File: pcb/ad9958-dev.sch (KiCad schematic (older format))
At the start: 88 parts, among them J2 5V, J3 OUT0, J4 OUT1, J5 HEAD-M10X2, U1 LM1117-1v8-SOT223, U2 LMH6714, U3 AD9958, U4 LMH6714, X1 25 MHz

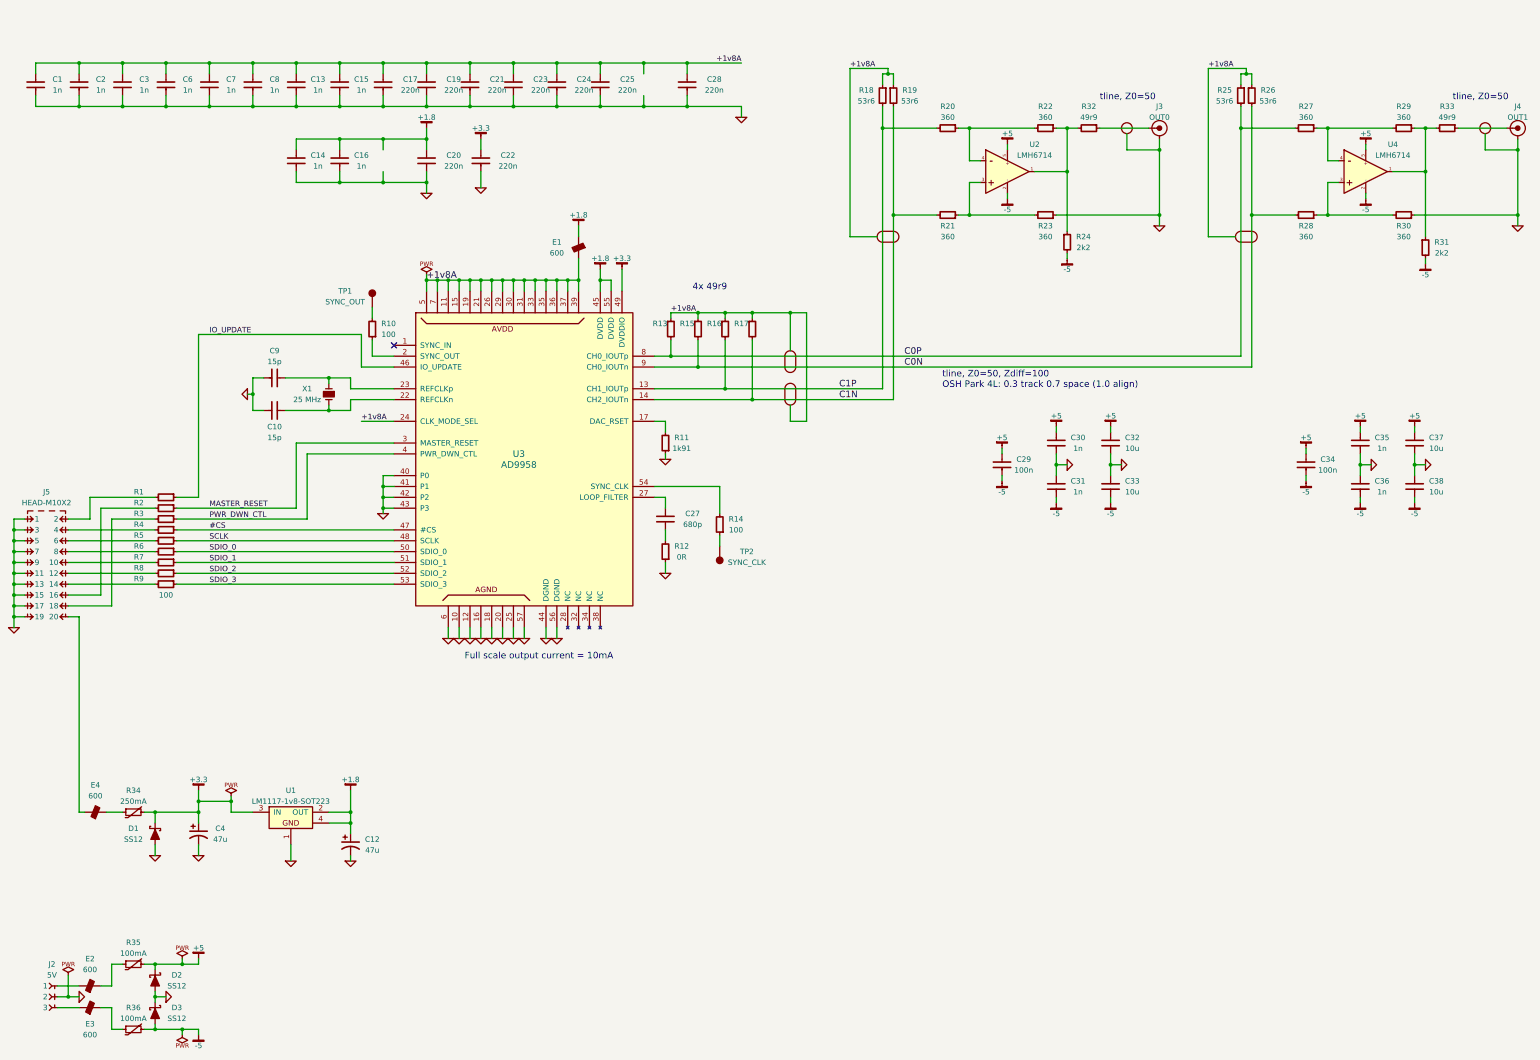
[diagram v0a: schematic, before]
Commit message: Schematic touchups
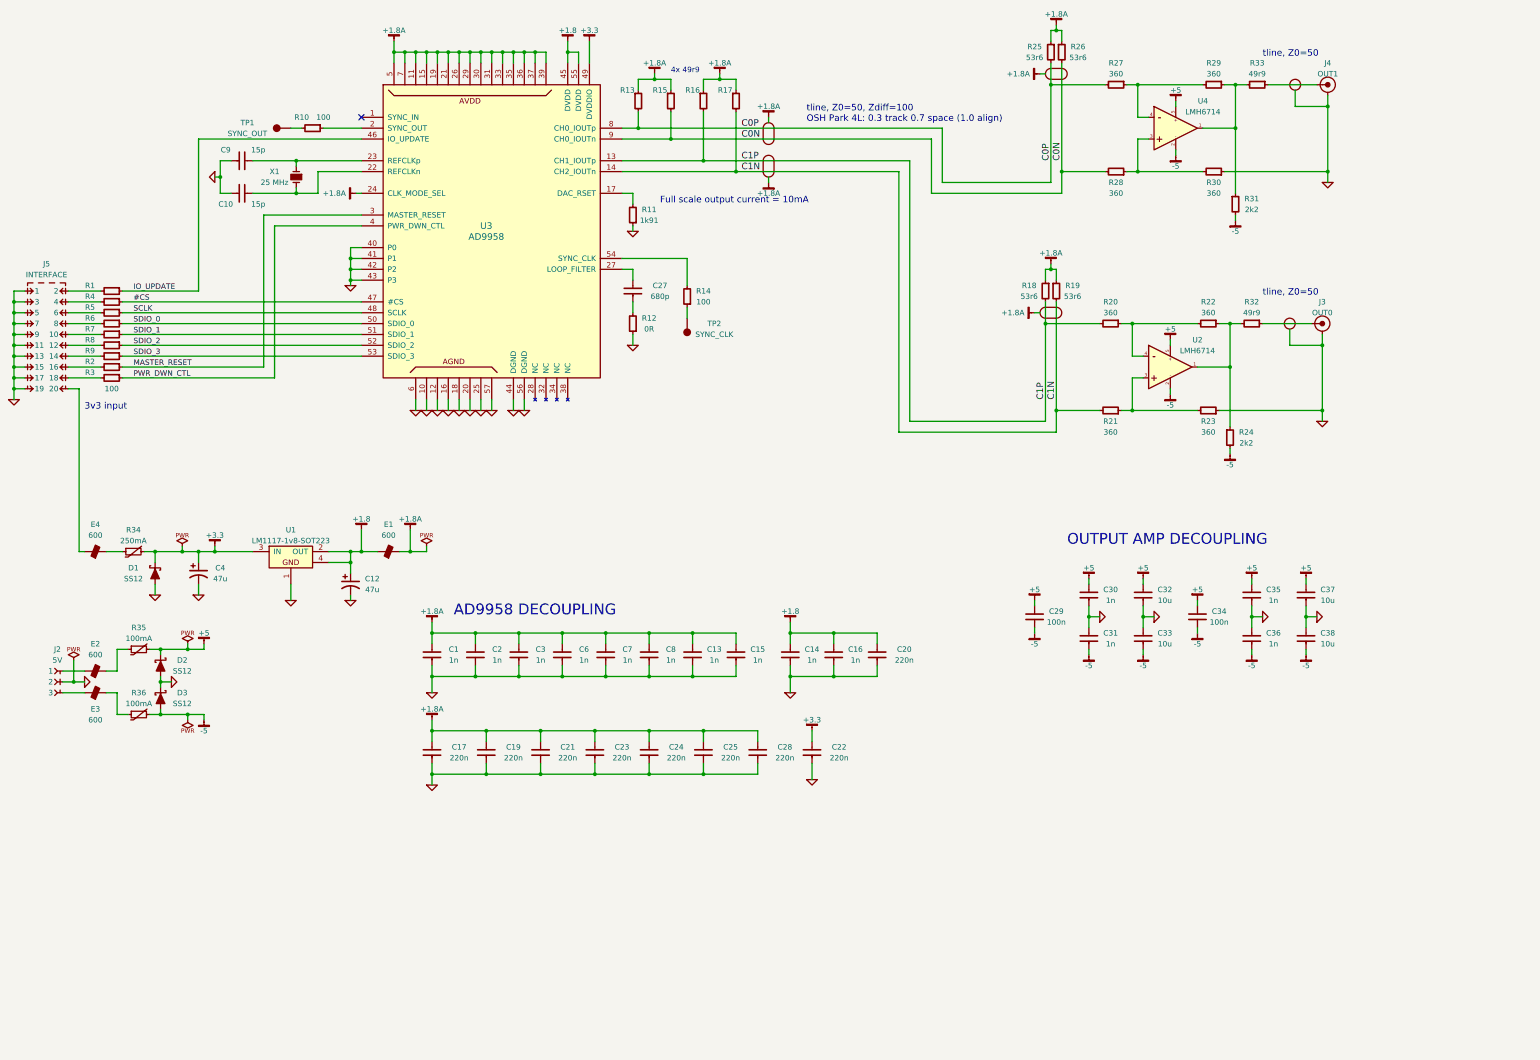
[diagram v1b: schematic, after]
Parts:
- J5: value HEAD-M10X2 -> INTERFACE
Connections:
- net +1v8A renamed +1.8A
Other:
- note added: "3v3 input"
- note added: "AD9958 DECOUPLING"
- note added: "OUTPUT AMP DECOUPLING"
- moved on the sheet: C1, C10, C12, C13, C14, C15, C16, C17, C19, C2, C20, C21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
